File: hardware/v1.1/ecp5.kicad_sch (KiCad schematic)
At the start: 8 parts, among them U1 ECP5U_12_CABGA256

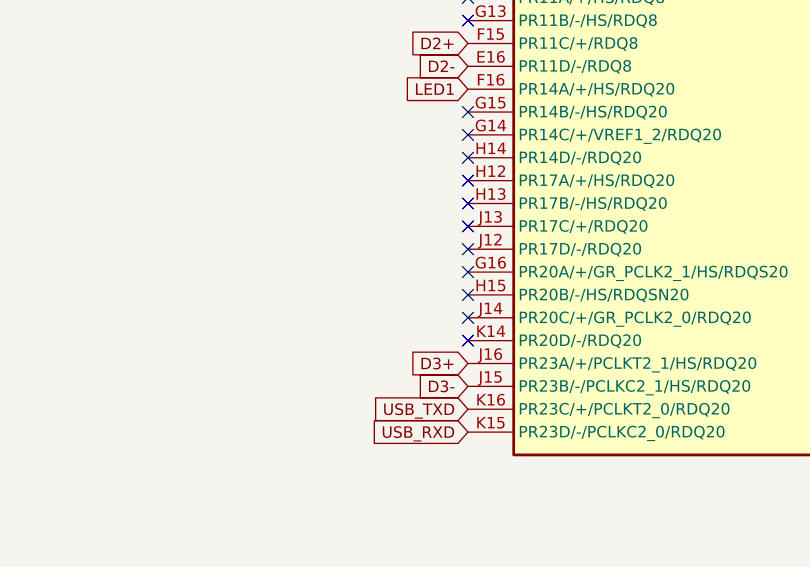
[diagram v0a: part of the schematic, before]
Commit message: Improvements of v1.1
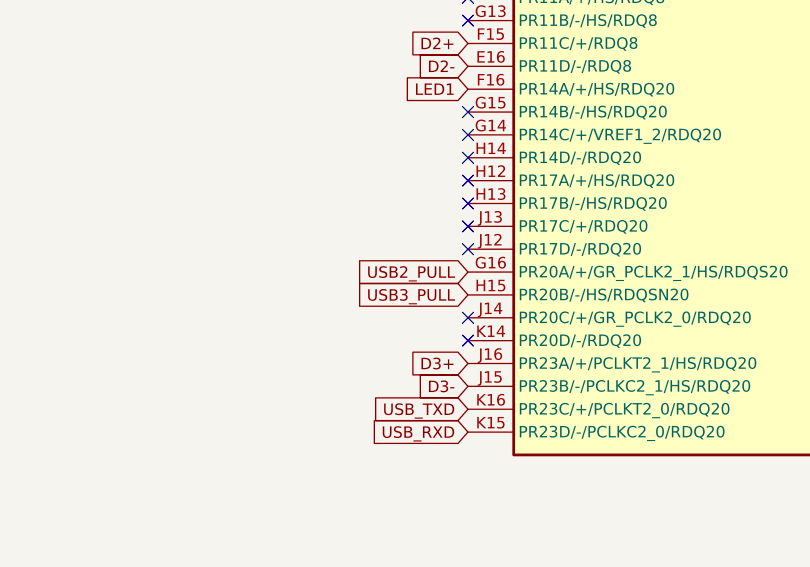
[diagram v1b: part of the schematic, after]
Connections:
- net USB2_PULL: now reaches U1.G16 (PR20A/+/GR_PCLK2_1/HS/RDQS20)
- net USB3_PULL: now reaches U1.H15 (PR20B/-/HS/RDQSN20)
- no-connect marks 50 -> 48
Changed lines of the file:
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@@
 		(title "Icepi zero")
 		(date "2025-05-12")
-		(rev "v1")
+		(rev "v1.1")
 		(company "Chengyin Yao (cheyao)")
 		(comment 1 "https://github.com/cheyao/icepi-zero")
@@
 	)
 	(no_connect
-		(at 214.63 85.09)
-	)
-	(no_connect
 		(at 31.75 163.83)
 	)
@@
 	(no_connect
 		(at 38.1 76.2)
-	)
-	(no_connect
-		(at 214.63 87.63)
 	)
 	(no_connect
@@
 		)
 	)
+	(global_label "USB2_PULL"
+		(shape input)
+		(at 214.63 85.09 180)
+		(fields_autoplaced yes)
+		(effects
+			(font
+				(size 1.27 1.27)
+			)
+			(justify right)
+		)
+		(property "Intersheetrefs" "${INTERSHEET_REFS}"
+			(at 201.001 85.09 0)
+			(effects
+				(font
+					(size 1.27 1.27)
+				)
+				(justify right)
+				(hide yes)
+			)
+		)
+	)
 	(global_label "GPIO_38"
 		(shape input)
@@
 			(effects
 				(font
+					(size 1.27 1.27)
+				)
+				(justify right)
+				(hide yes)
+			)
+		)
+	)
+	(global_label "USB3_PULL"
+		(shape input)
+		(at 214.63 87.63 180)
+		(fields_autoplaced yes)
+		(effects
+			(font
+				(size 1.27 1.27)
+			)
+			(justify right)
+		)
+		(property "Intersheetrefs" "${INTERSHEET_REFS}"
+			(at 201.001 87.63 0)
+			(effects
+				(font
